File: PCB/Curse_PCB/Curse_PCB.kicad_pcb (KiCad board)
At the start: 2 copper layers, 54.2 x 30.2 mm, 47 parts

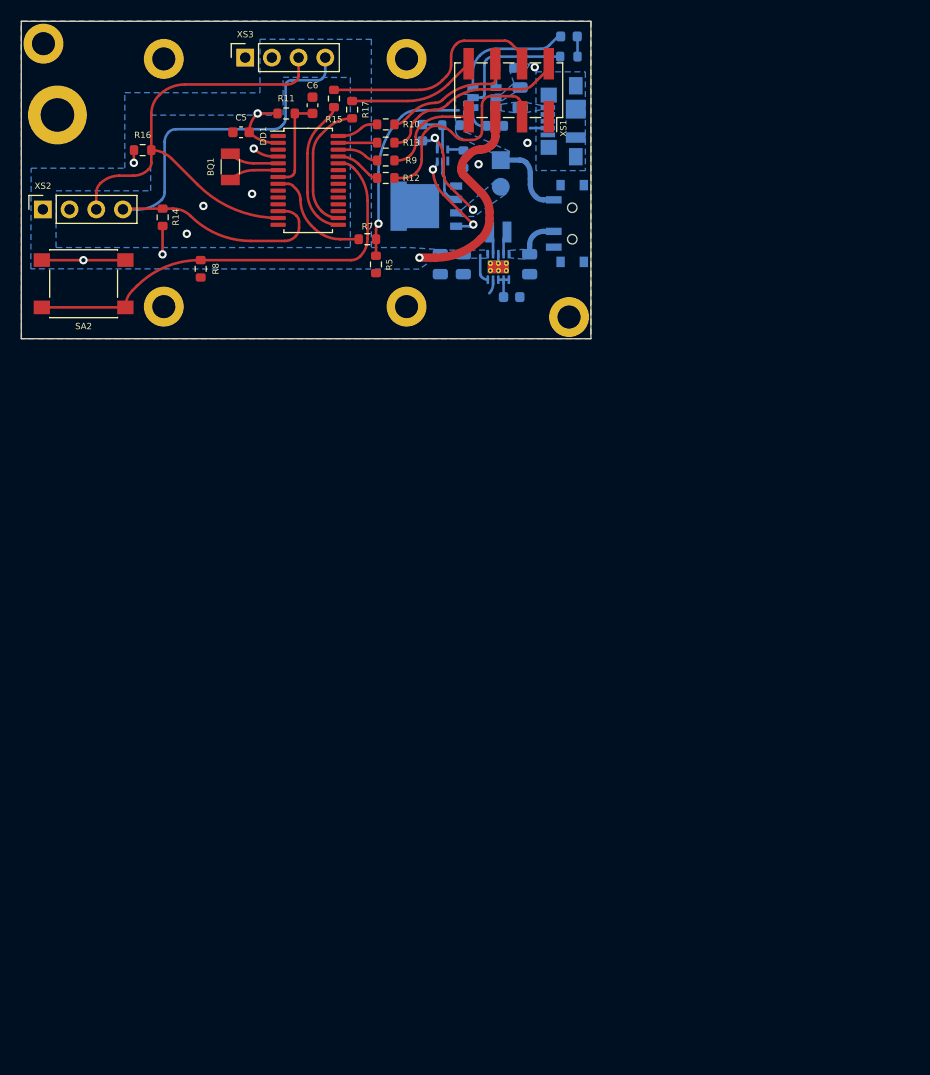
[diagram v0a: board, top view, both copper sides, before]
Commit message: almost done
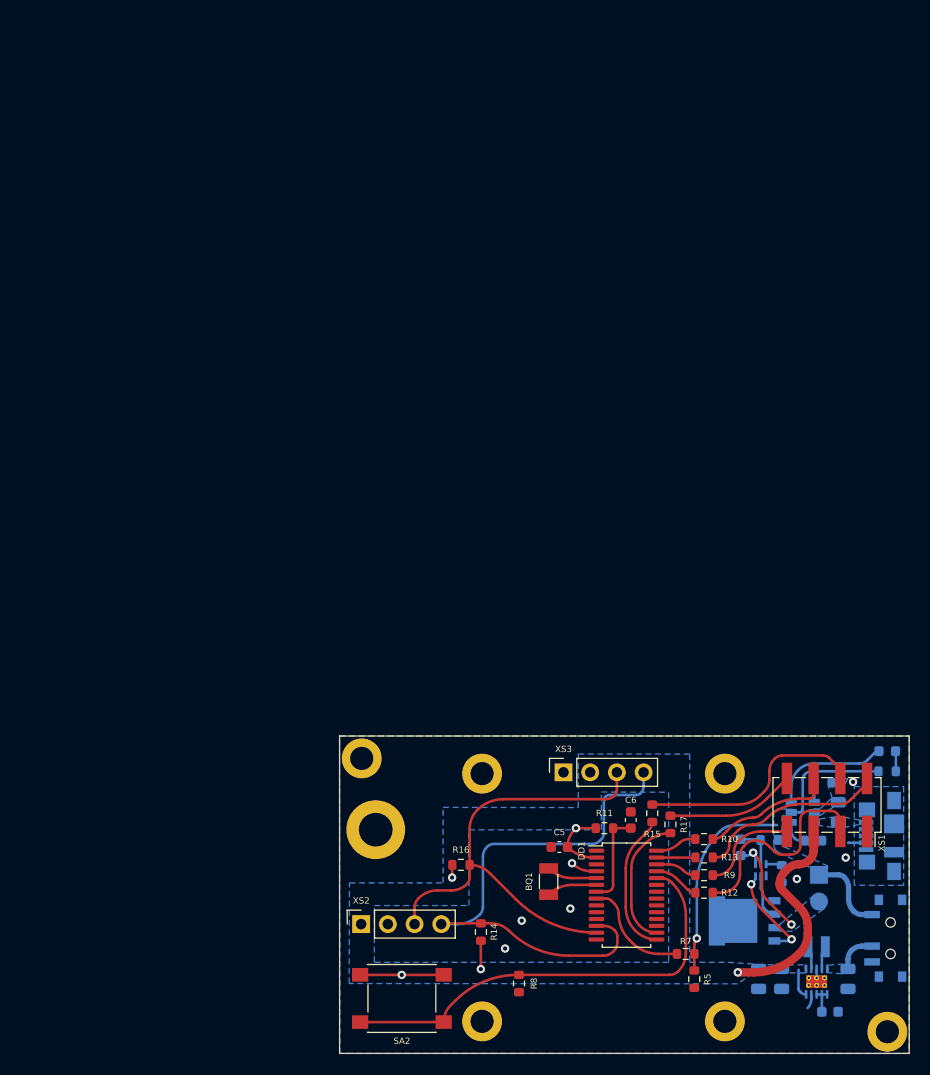
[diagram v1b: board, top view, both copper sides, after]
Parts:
- moved C7 74.4 mm to (124.2, 132.0)
- moved C8 74.4 mm to (126.4, 132.0)
- moved R7 74.4 mm to (117.3, 129.6)
- moved C2 74.4 mm to (131.8, 116.1)
- moved C3 74.4 mm to (132.7, 132.0)
- moved C4 74.4 mm to (131.0, 135.1)
- moved GB1 74.4 mm to (130.0, 122.1)
- moved HL1 74.4 mm to (136.5, 110.3)
- moved L1 74.4 mm to (131.0, 129.9)
- moved R10 74.4 mm to (119.1, 118.7)
- moved R12 74.4 mm to (119.1, 123.8)
- moved R13 74.4 mm to (119.1, 120.4)
- moved R17 74.4 mm to (115.9, 117.3)
- moved R2 74.4 mm to (130.4, 113.3)
- moved R8 74.4 mm to (101.4, 132.4)
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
